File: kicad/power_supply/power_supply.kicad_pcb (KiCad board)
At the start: 2 copper layers, 105.7 x 48 mm, 23 parts, among them J1 AC1, J2 GND, J3 CT, J4 AC2, J5 V-, J6 V+

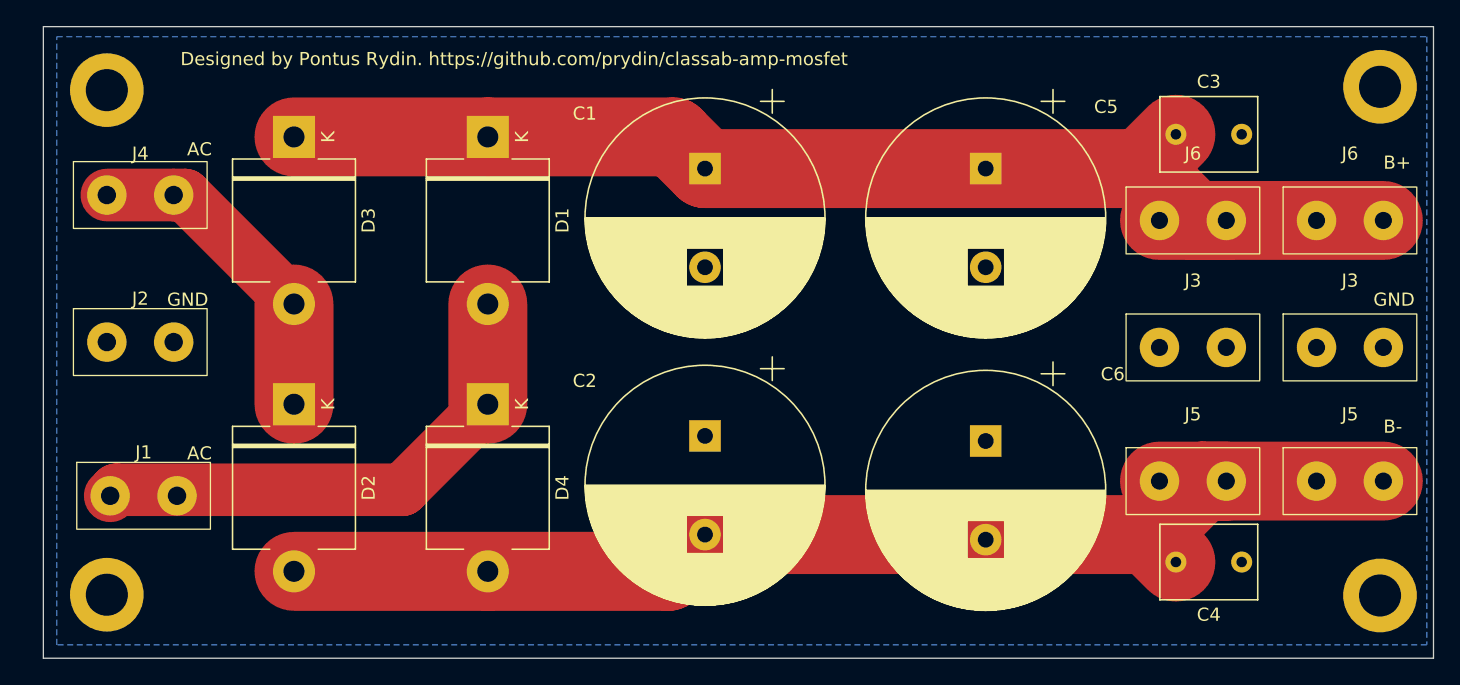
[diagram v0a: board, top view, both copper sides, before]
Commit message: Public release candidate
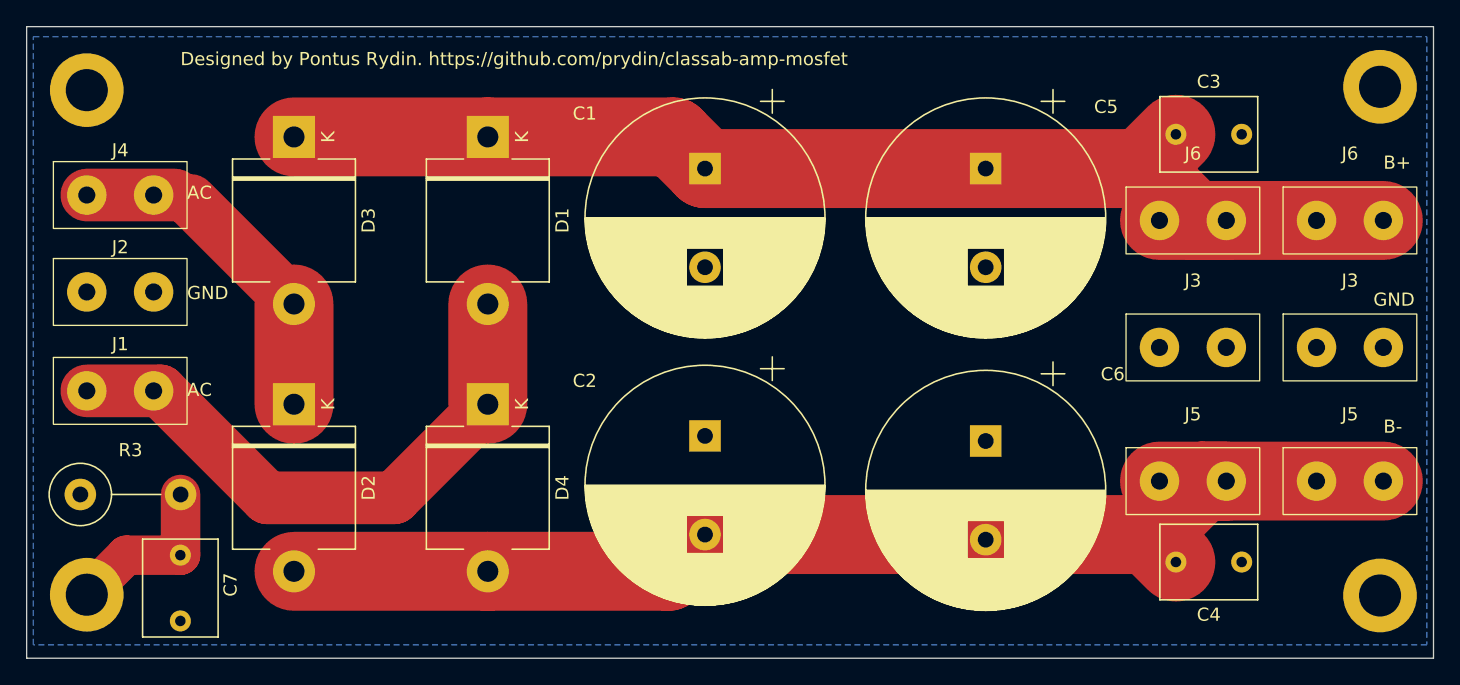
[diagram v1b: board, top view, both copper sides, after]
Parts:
- added C7: 100n, Capacitor_THT:C_Rect_L7.2mm_W5.5mm_P5.00mm_FKS2_FKP2_MKS2_MKP2, F.Cu at (74.4, 106.6)
- added R3: 220, Resistor_THT:R_Axial_DIN0414_L11.9mm_D4.5mm_P7.62mm_Vertical, F.Cu at (66.8, 97.0)
- moved J1 8.17 mm to (69.8, 84.1)
- moved J2 4.10 mm to (69.8, 76.6)
- moved J4 1.52 mm to (69.8, 69.2)
- moved REF** 1.52 mm to (67.3, 66.3)
- moved REF** 1.52 mm to (67.3, 104.6)
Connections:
- REF** pad 1: GND -> GNDPWR
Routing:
- net GNDPWR: track 0.00 -> 13.0 mm
- net /AC1: track 39.2 -> 44.4 mm
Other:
- board size 105.7 x 48 mm -> 106.9 x 48 mm
